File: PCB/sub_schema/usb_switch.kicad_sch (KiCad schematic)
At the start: 15 parts, among them J1 USB3_A, U2 NCP1117-1.5_SOT223, U4 HD3SS6126RUAR, U6 TPS628437DRL, U9 TPS628437DRL

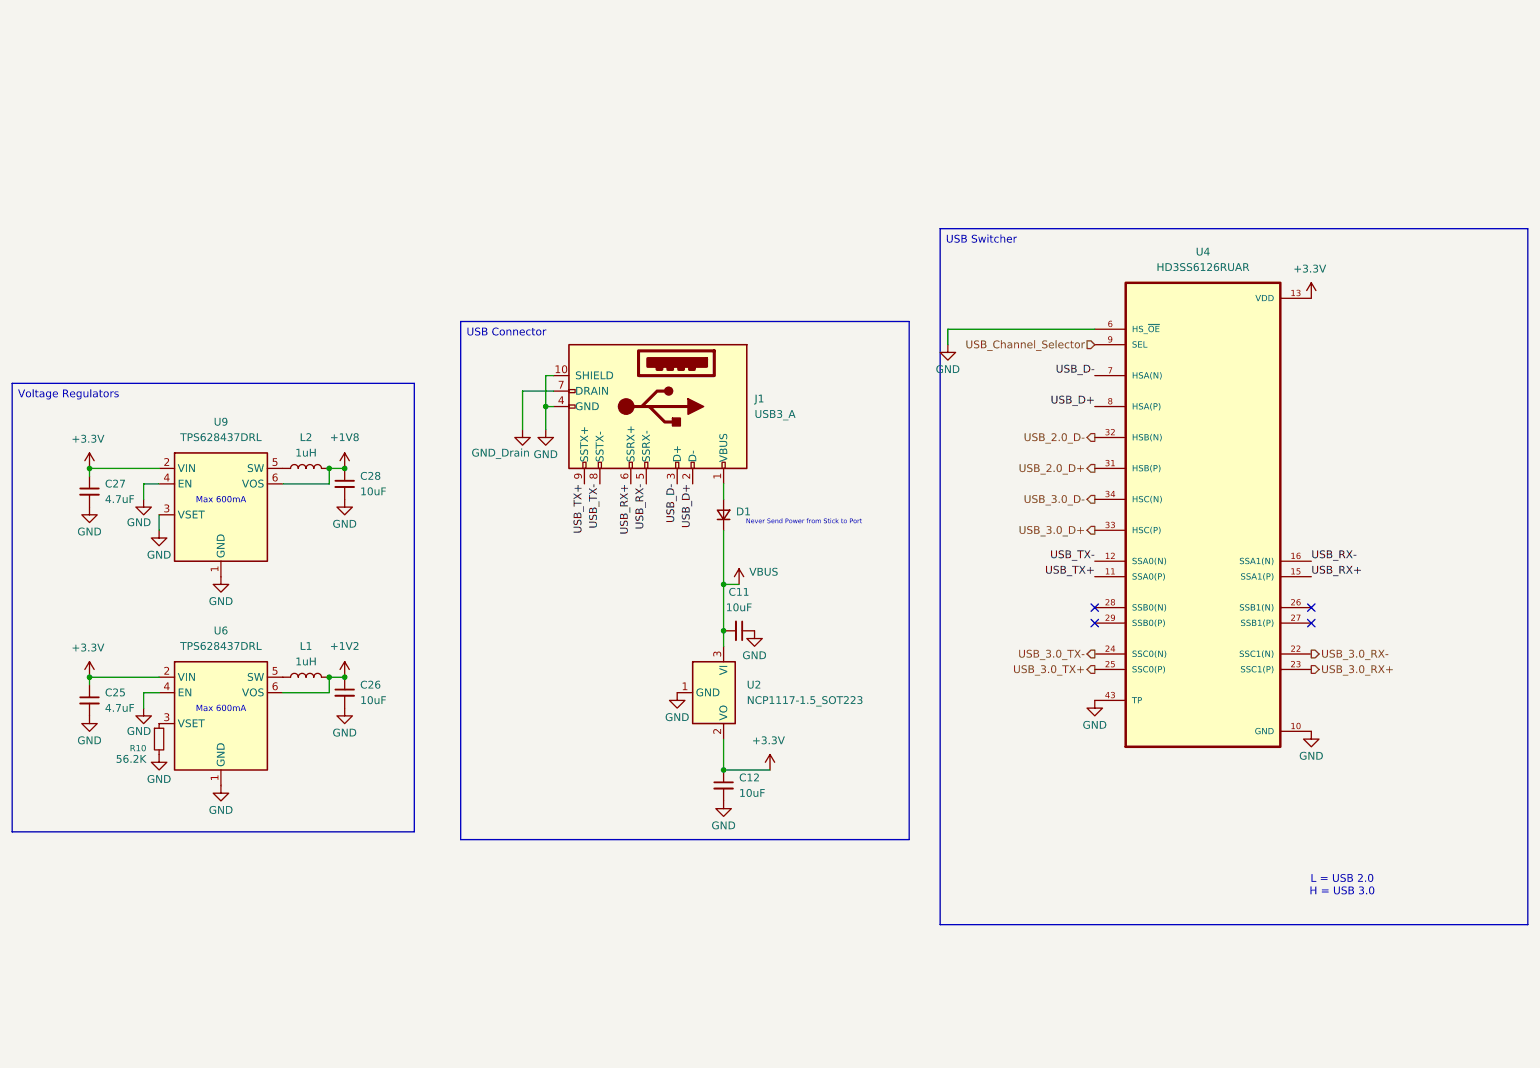
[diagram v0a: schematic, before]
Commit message: worked on BOM
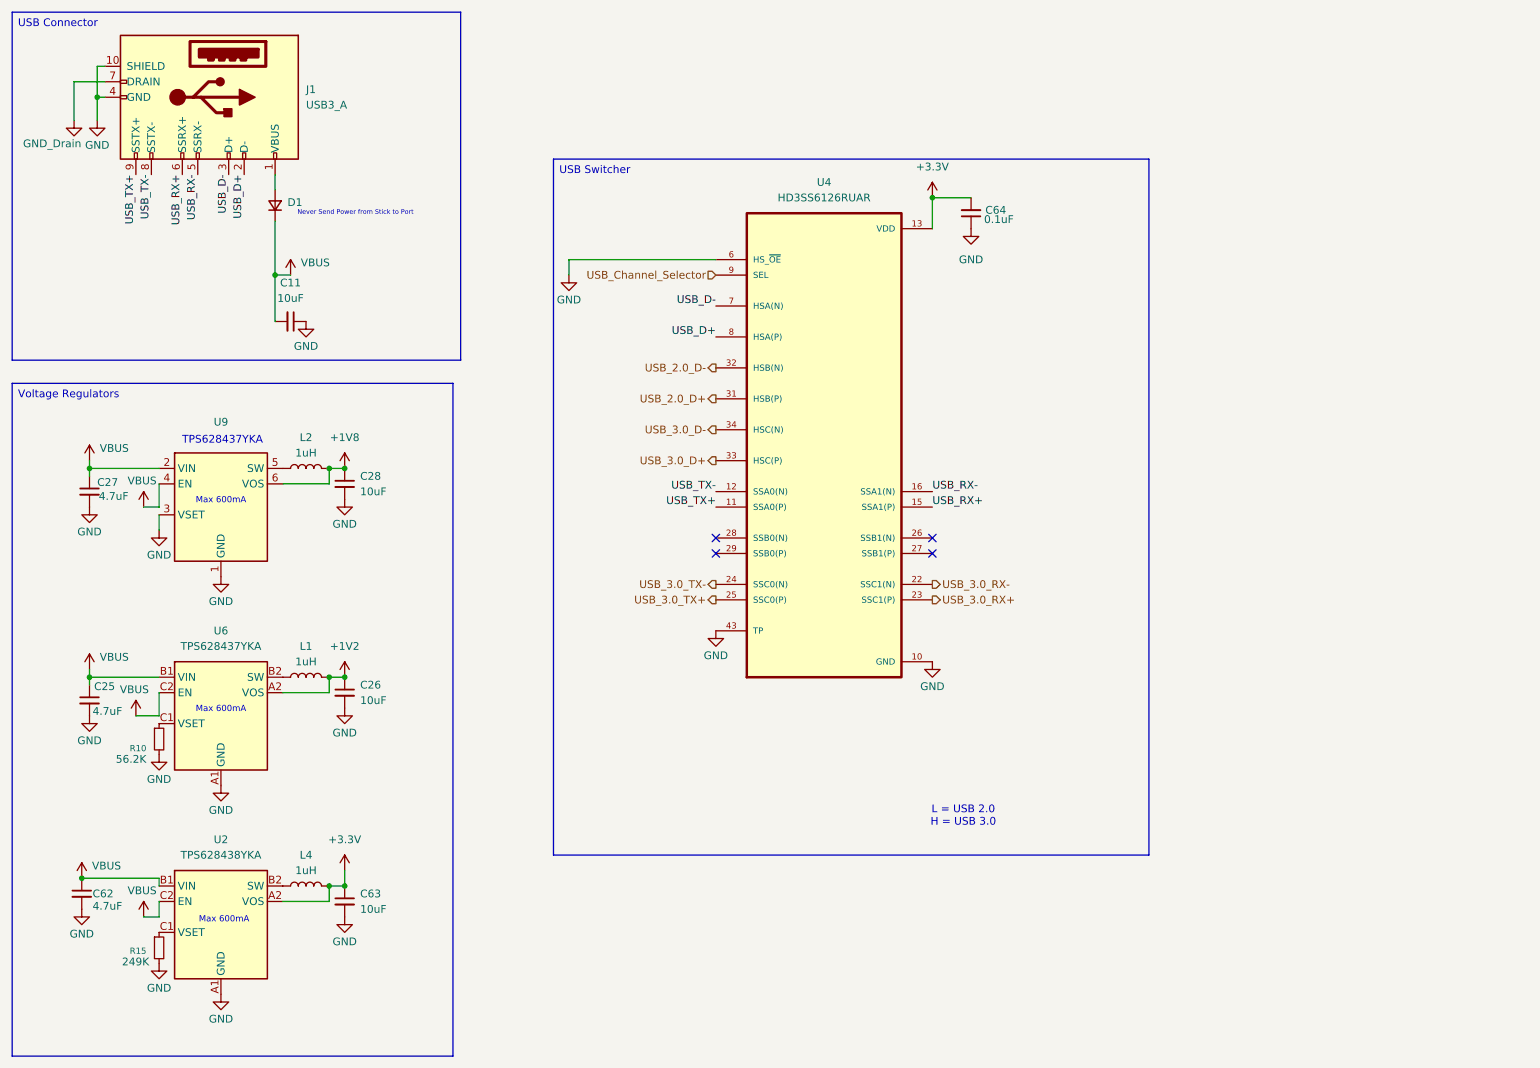
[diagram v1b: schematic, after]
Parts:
- removed C12: 10uF, symbol Device:C_Small
- removed U2: NCP1117-1.5_SOT223, symbol Regulator_Linear:NCP1117-1.5_SOT223
- added C62: 4.7uF, Capacitor_SMD:C_0402_1005Metric, symbol Device:C_Small
- added C63: 10uF, Capacitor_SMD:C_0402_1005Metric, symbol Device:C_Small
- added C64: 0.1uF, Capacitor_SMD:C_0201_0603Metric, symbol Device:C_Small
- added L4: 1uH, symbol Device:L
- added R15: 249K, Resistor_SMD:R_0201_0603Metric, symbol Device:R_Small
- added U2: TPS628438YKA, symbol Regulator_Switching:TPS628438YKA
- C11, C25, C26, C27, C28: footprint (none) -> Capacitor_SMD:C_0402_1005Metric
- R10: footprint (none) -> Resistor_SMD:R_0201_0603Metric
- U6: value TPS628437DRL -> TPS628437YKA; symbol Regulator_Switching:TPS628437DRL -> Regulator_Switching:TPS628437YKA
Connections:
- net +1V2: now also U6.A2 (VOS); no longer U6.6 (VOS)
- net +3.3V: now also C63.1, C64.2, L4.2, U2.A2 (VOS); no longer C25.1, C27.1, U6.2 (VIN), U9.2 (VIN)
- net GND: now also U6.A1 (GND), C62.2, C63.2, C64.1, R15.2, U2.A1 (GND); no longer U6.1 (GND), U6.4 (EN), U9.4 (EN)
- net VBUS: now also C25.1, C27.1, U6.B1 (VIN), U6.C2 (EN), U9.2 (VIN), U9.4 (EN), C62.1, U2.B1 (VIN), U2.C2 (EN)
- net at R10.1: now also U6.C1 (VSET); no longer U6.3 (VSET)
- net at L1.1: now also U6.B2 (SW); no longer U6.5 (SW)
- new net: L4.1, U2.B2 (SW)
- new net: R15.1, U2.C1 (VSET)
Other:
- note added: "TPS628437YKA"
- moved on the sheet: C11, D1, J1, U4
